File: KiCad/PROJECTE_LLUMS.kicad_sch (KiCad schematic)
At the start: 0 parts

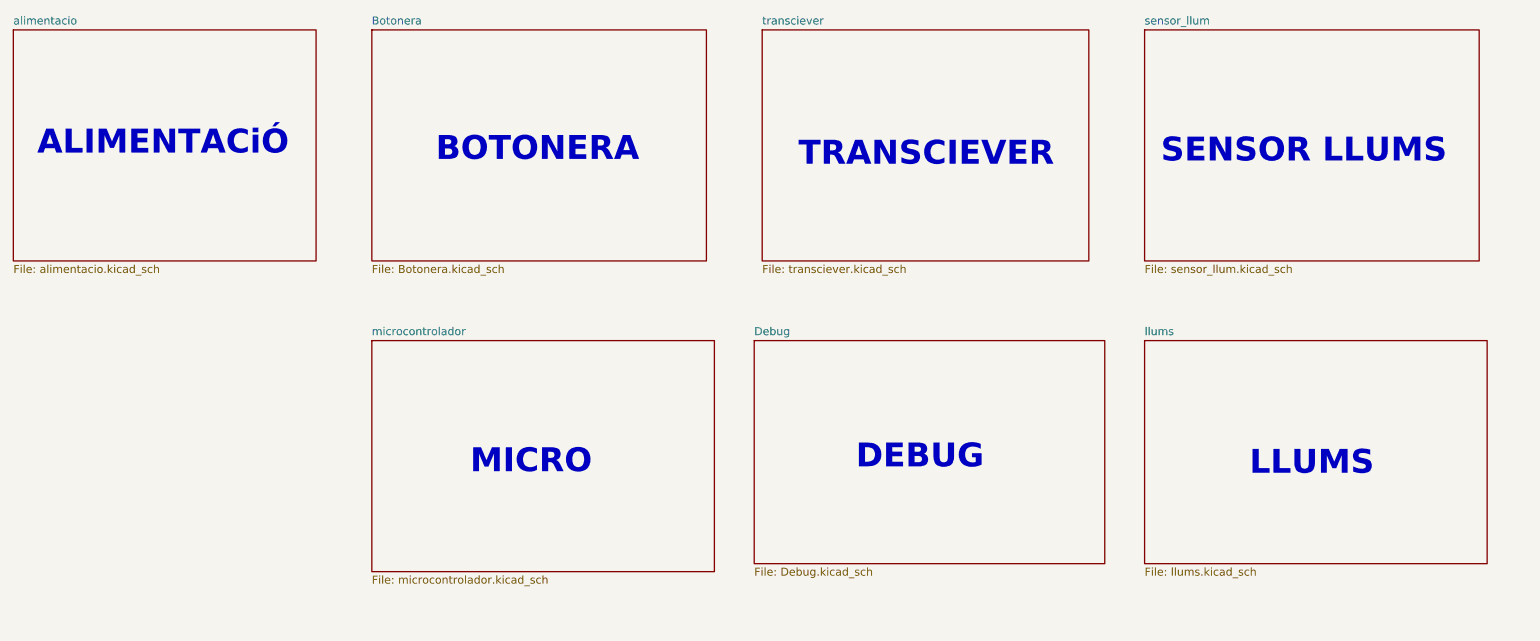
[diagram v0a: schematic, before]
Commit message: ERC i footprints
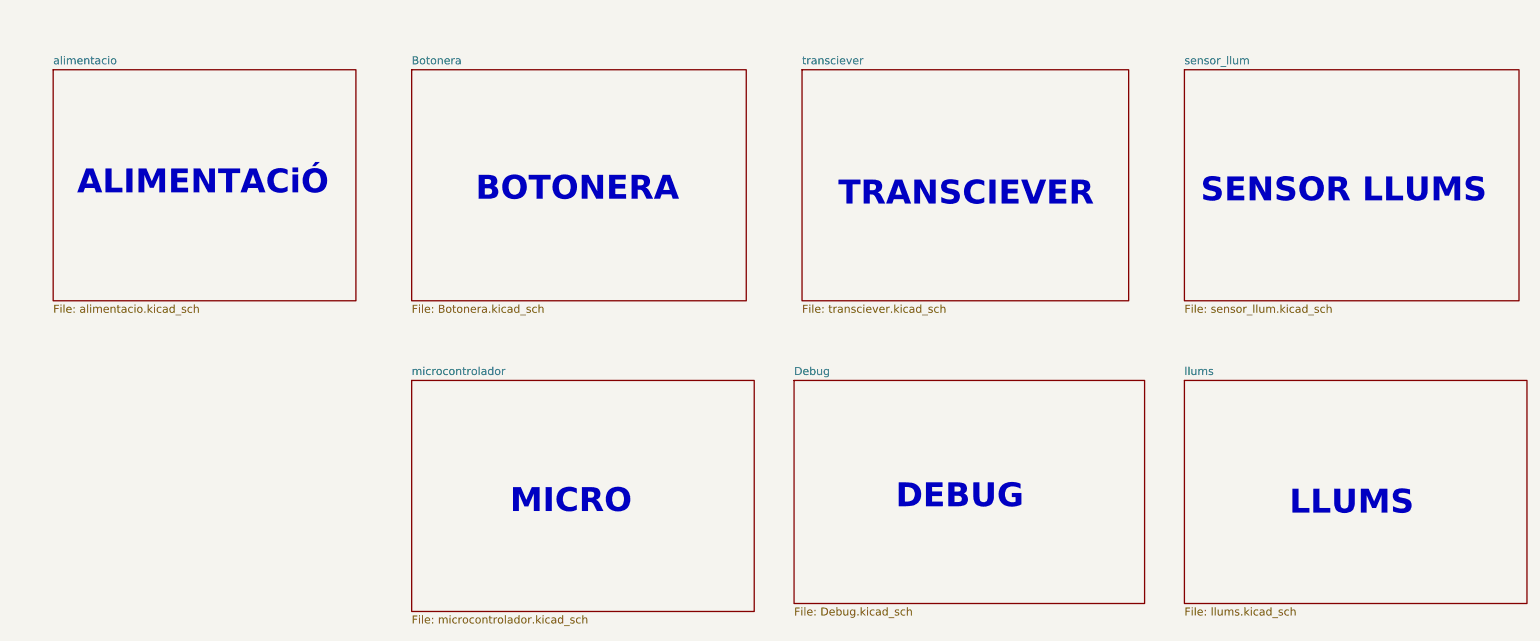
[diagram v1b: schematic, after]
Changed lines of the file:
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@@
 	(text "DEBUG\n"
 		(exclude_from_sim no)
-		(at 168.656 88.392 0)
+		(at 175.006 94.742 0)
 		(effects
 			(font
@@
 	(text "ALIMENTACiÓ"
 		(exclude_from_sim no)
-		(at 48.006 38.354 0)
+		(at 54.356 44.704 0)
 		(effects
 			(font
@@
 	(text "MICRO"
 		(exclude_from_sim no)
-		(at 106.68 89.154 0)
+		(at 113.03 95.504 0)
 		(effects
 			(font
@@
 	(text "LLUMS\n"
 		(exclude_from_sim no)
-		(at 231.14 89.408 0)
+		(at 237.49 95.758 0)
 		(effects
 			(font
@@
 	(text "TRANSCIEVER\n"
 		(exclude_from_sim no)
-		(at 169.672 40.132 0)
+		(at 176.022 46.482 0)
 		(effects
 			(font
@@
 	(text "BOTONERA\n"
 		(exclude_from_sim no)
-		(at 107.696 39.37 0)
+		(at 114.046 45.72 0)
 		(effects
 			(font
@@
 	(text "SENSOR LLUMS\n"
 		(exclude_from_sim no)
-		(at 229.87 39.624 0)
-		(effects
-			(font
-				(size 3.81 3.81)
-				(thickness 0.762)
-				(bold yes)
-			)
-		)
-	)
-	(sheet
-		(at 204.47 69.85)
+		(at 236.22 45.974 0)
+		(effects
+			(font
+				(size 3.81 3.81)
+				(thickness 0.762)
+				(bold yes)
+			)
+		)
+	)
+	(sheet
+		(at 210.82 76.2)
 		(size 54.61 35.56)
 		(exclude_from_sim no)
@@
 		)
 		(property "Sheetname" "llums"
-			(at 204.47 69.1384 0)
+			(at 210.82 75.4884 0)
 			(effects
 				(font
@@
 		)
 		(property "Sheetfile" "llums.kicad_sch"
-			(at 204.47 105.9946 0)
+			(at 210.82 112.3446 0)
 			(effects
 				(font
@@
 	)
 	(sheet
-		(at 204.47 20.32)
+		(at 210.82 26.67)
 		(size 53.34 36.83)
 		(exclude_from_sim no)
@@
 		)
 		(property "Sheetname" "sensor_llum"
-			(at 204.47 19.6084 0)
+			(at 210.82 25.9584 0)
 			(effects
 				(font
@@
 		)
 		(property "Sheetfile" "sensor_llum.kicad_sch"
-			(at 204.47 57.7346 0)
+			(at 210.82 64.0846 0)
 			(effects
 				(font
@@
 	)
 	(sheet
-		(at 81.28 69.85)
+		(at 87.63 76.2)
 		(size 54.61 36.83)
 		(exclude_from_sim no)
@@
 		)
 		(property "Sheetname" "microcontrolador"
-			(at 81.28 69.1384 0)
+			(at 87.63 75.4884 0)
 			(effects
 				(font
@@
 		)
 		(property "Sheetfile" "microcontrolador.kicad_sch"
-			(at 81.28 107.2646 0)
+			(at 87.63 113.6146 0)
 			(effects
 				(font
@@
 	)
 	(sheet
-		(at 81.28 20.32)
+		(at 87.63 26.67)
 		(size 53.34 36.83)
 		(exclude_from_sim no)
@@
 		)
 		(property "Sheetname" "Botonera"
-			(at 81.28 19.6084 0)
+			(at 87.63 25.9584 0)
 			(effects
 				(font
@@
 		)
 		(property "Sheetfile" "Botonera.kicad_sch"
-			(at 81.28 57.7346 0)
+			(at 87.63 64.0846 0)
 			(effects
 				(font
@@
 	)
 	(sheet
-		(at 24.13 20.32)
+		(at 30.48 26.67)
 		(size 48.26 36.83)
 		(exclude_from_sim no)
@@
 		)
 		(property "Sheetname" "alimentacio"
-			(at 24.13 19.6084 0)
+			(at 30.48 25.9584 0)
 			(effects
 				(font
@@
 		)
 		(property "Sheetfile" "alimentacio.kicad_sch"
-			(at 24.13 57.7346 0)
+			(at 30.48 64.0846 0)
 			(effects
 				(font
@@
 	)
 	(sheet
-		(at 142.24 69.85)
+		(at 148.59 76.2)
 		(size 55.88 35.56)
 		(exclude_from_sim no)
@@
 		)
 		(property "Sheetname" "Debug"
-			(at 142.24 69.1384 0)
+			(at 148.59 75.4884 0)
 			(effects
 				(font
@@
 		)
 		(property "Sheetfile" "Debug.kicad_sch"
-			(at 142.24 105.9946 0)
+			(at 148.59 112.3446 0)
 			(effects
 				(font
@@
 	)
 	(sheet
-		(at 143.51 20.32)
+		(at 149.86 26.67)
 		(size 52.07 36.83)
 		(exclude_from_sim no)
@@
 		)
 		(property "Sheetname" "transciever"
-			(at 143.51 19.6084 0)
+			(at 149.86 25.9584 0)
 			(effects
 				(font
@@
 		)
 		(property "Sheetfile" "transciever.kicad_sch"
-			(at 143.51 57.7346 0)
-			(effects
-				(font
+			(at 149.86 64.0846 0)
+			(effects
+				(font
